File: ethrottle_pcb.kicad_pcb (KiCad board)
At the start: 2 copper layers, 59 x 48 mm, 59 parts, among them J1 ATM15-08PA-BM02, Q1 ZXTR2105F-7, U1 MCP6004, U2 MCP6004, U3 MCP6004, U4 UB2-5NUN

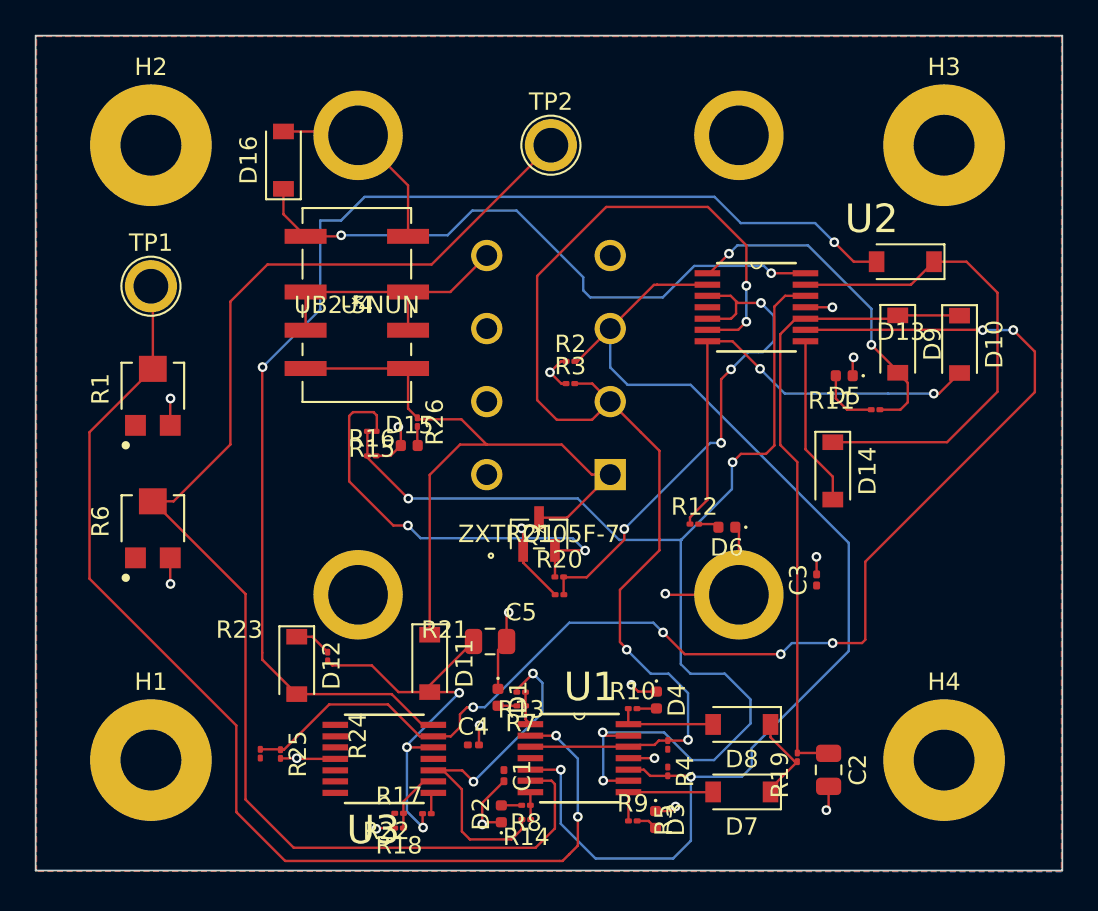
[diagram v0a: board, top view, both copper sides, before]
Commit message: silkscreen
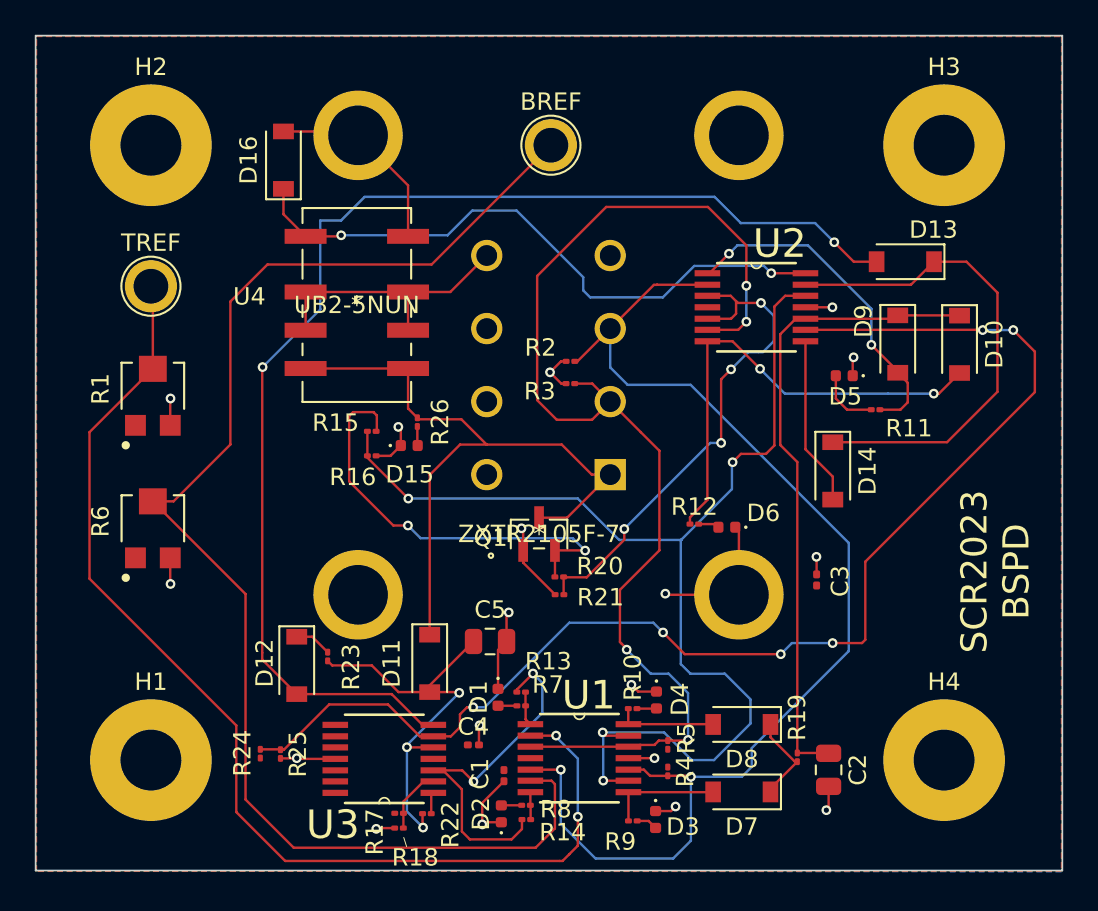
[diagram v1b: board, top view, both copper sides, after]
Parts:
- renumbered TP2 to BREF, TP1 to TREF
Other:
- board text added: "SCR2023 BSPD"
- board text added: "\"

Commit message: silkscreen
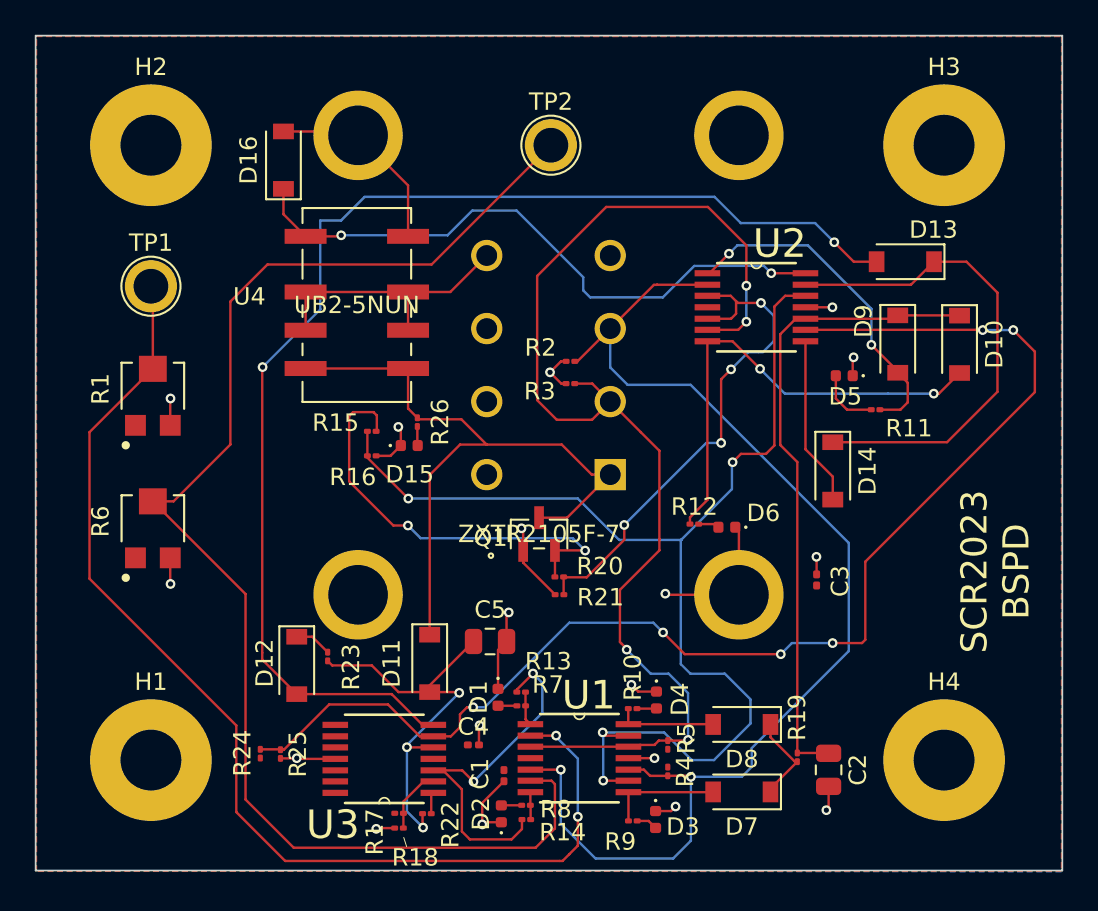
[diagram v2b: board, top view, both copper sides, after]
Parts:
- renumbered TREF to TP1, BREF to TP2
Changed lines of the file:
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@@
       (effects (font (size 1 1) (thickness 0.15)))
     )
-    (fp_text user "*" (at 0 0) (layer "F.SilkS")
+    (fp_text user "*" (at 0 0) (layer "F.SilkS") hide
       (effects (font (size 1 1) (thickness 0.15)))
     )
@@
     (property "Sheetname" "")
     (attr exclude_from_pos_files)
-    (fp_text reference "BREF" (at 0 -2.498) (layer "F.SilkS")
+    (fp_text reference "TP2" (at 0 -2.498) (layer "F.SilkS")
       (effects (font (size 1 1) (thickness 0.15)))
     )
@@
       (effects (font (size 1 1) (thickness 0.15)))
     )
-    (fp_text user "*" (at 0 0) (layer "F.SilkS")
+    (fp_text user "*" (at 0 0) (layer "F.SilkS") hide
       (effects (font (size 1 1) (thickness 0.15)))
     )
@@
     (property "Sheetname" "")
     (attr exclude_from_pos_files)
-    (fp_text reference "TREF" (at 0 -2.498) (layer "F.SilkS")
+    (fp_text reference "TP1" (at 0 -2.498) (layer "F.SilkS")
       (effects (font (size 1 1) (thickness 0.15)))
     )
@@
   (segment (start 129.8394 77.4894) (end 129.8394 71.2758) (width 0.1397) (layer "F.Cu") (net 32))
   (segment (start 131.41 79.06) (end 129.8394 77.4894) (width 0.1397) (layer "F.Cu") (net 32))
-  (segment (start 131.3958 80.3658) (end 131.41 80.38) (width 0.1397) (layer "F.Cu") (net 32))
-  (segment (start 131.41 80.38) (end 131.41 79.06) (width 0.1397) (layer "F.Cu") (net 32))
+  (segment (start 131.41 79.06) (end 131.41 80.38) (width 0.1397) (layer "F.Cu") (net 32))
   (segment (start 107.52 77.25) (end 107.54 77.27) (width 0.1397) (layer "F.Cu") (net 33))
   (segment (start 107.52 76.175) (end 107.52 77.25) (width 0.1397) (layer "F.Cu") (net 33))
@@
   (segment (start 117.26 84.85) (end 115.9525 84.85) (width 0.1397) (layer "F.Cu") (net 34))
   (segment (start 115.93 84.8275) (end 115.93 85.8325) (width 0.1397) (layer "F.Cu") (net 34))
-  (segment (start 119.42 82.07) (end 119.42 82.69) (width 0.1397) (layer "F.Cu") (net 34))
+  (segment (start 119.42 82.69) (end 119.42 81.84) (width 0.1397) (layer "F.Cu") (net 34))
   (segment (start 125.85 68.97) (end 125.5396 68.6596) (width 0.1397) (layer "F.Cu") (net 34))
   (segment (start 127.28 69.07) (end 125.95 69.07) (width 0.1397) (layer "F.Cu") (net 34))
@@
   (segment (start 115.9525 84.85) (end 115.93 84.8275) (width 0.1397) (layer "F.Cu") (net 34))
   (via (at 124.99 77.12) (size 0.56) (drill 0.3) (layers "F.Cu" "B.Cu") (net 34))
+  (via (at 119.42 81.84) (size 0.56) (drill 0.3) (layers "F.Cu" "B.Cu") (net 34))
   (via (at 127.28 69.07) (size 0.56) (drill 0.3) (layers "F.Cu" "B.Cu") (net 34))
-  (via (at 119.42 82.07) (size 0.56) (drill 0.3) (layers "F.Cu" "B.Cu") (net 34))
   (via (at 125.56 72.89) (size 0.56) (drill 0.3) (layers "F.Cu" "B.Cu") (net 34))
-  (segment (start 119.42 82.07) (end 124.37 77.12) (width 0.1397) (layer "B.Cu") (net 34))
-  (segment (start 124.37 77.12) (end 124.99 77.12) (width 0.1397) (layer "B.Cu") (net 34))
-  (segment (start 119.39 82.07) (end 119.42 82.07) (width 0.1397) (layer "B.Cu") (net 34))
+  (segment (start 119.42 81.84) (end 124.14 77.12) (width 0.1397) (layer "B.Cu") (net 34))
+  (segment (start 124.14 77.12) (end 124.99 77.12) (width 0.1397) (layer "B.Cu") (net 34))
   (segment (start 126.55 71.9) (end 127.15 71.9) (width 0.1397) (layer "B.Cu") (net 34))
   (segment (start 125.56 72.89) (end 126.55 71.9) (width 0.1397) (layer "B.Cu") (net 34))
